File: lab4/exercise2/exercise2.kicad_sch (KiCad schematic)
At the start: 10 parts, among them J1 Conn_01x02_Male, U1 NE555D

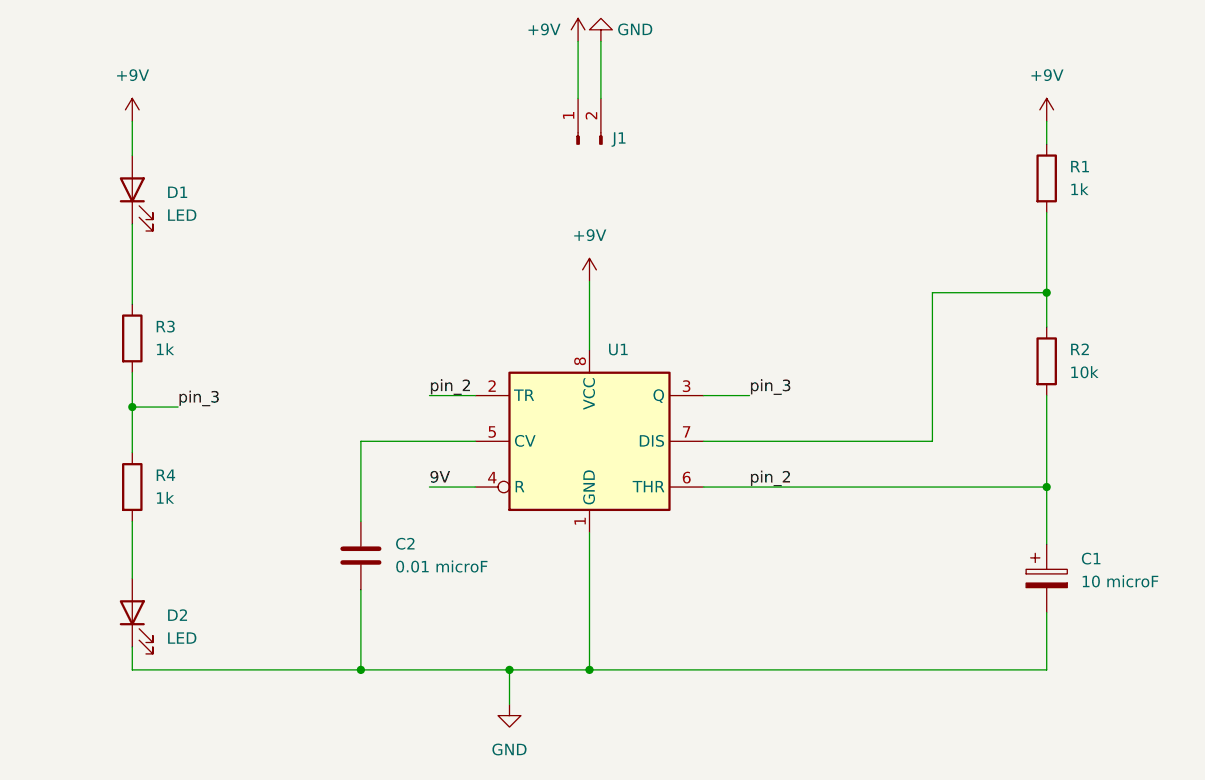
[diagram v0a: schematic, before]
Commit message: PCB layout
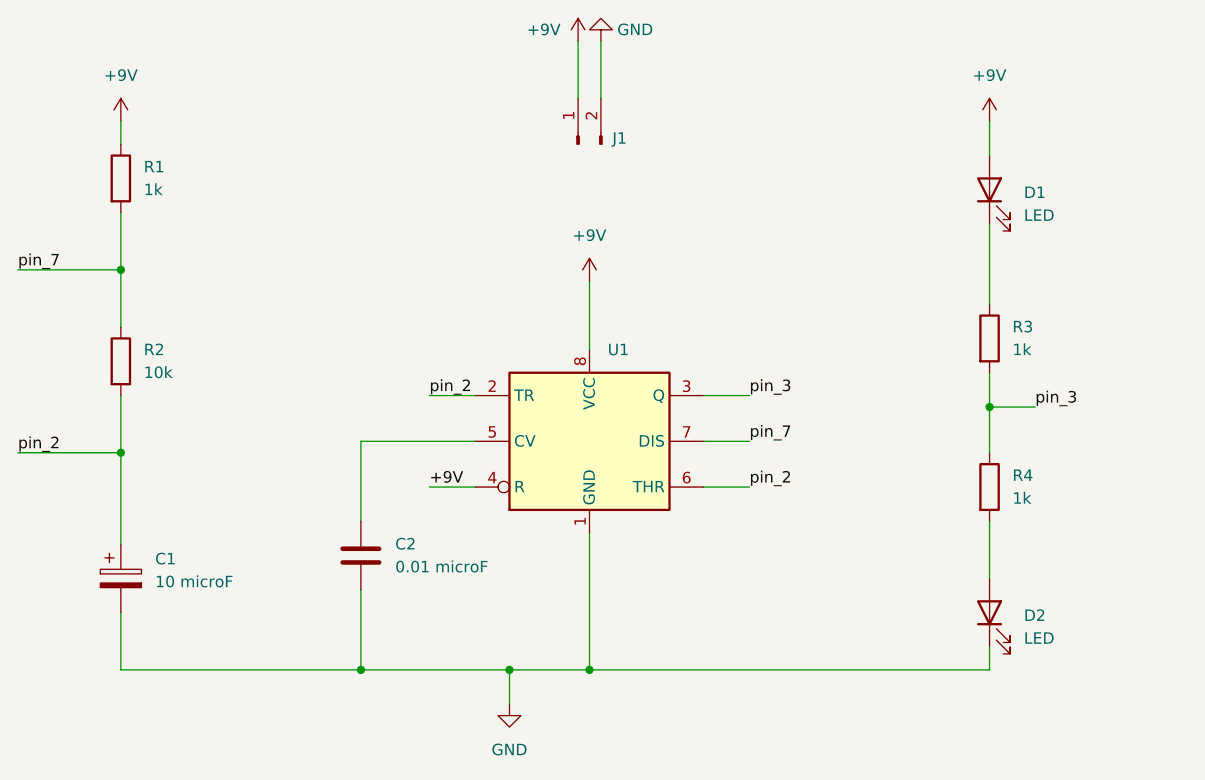
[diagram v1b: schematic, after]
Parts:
- C1: footprint (none) -> Capacitor_Tantalum_SMD:CP_EIA-3216-18_Kemet-A_Pad1.58x1.35mm_HandSolder
- C2: footprint (none) -> Capacitor_SMD:C_0805_2012Metric_Pad1.18x1.45mm_HandSolder
- D1, D2: footprint (none) -> LED_SMD:LED_1206_3216Metric_Pad1.42x1.75mm_HandSolder
- J1: footprint (none) -> TerminalBlock:TerminalBlock_bornier-2_P5.08mm
- R1, R2, R3, R4: footprint (none) -> Resistor_SMD:R_0805_2012Metric_Pad1.20x1.40mm_HandSolder
- U1: footprint Package_SO:SOIC-8_3.9x4.9mm_P1.27mm -> Package_SO:SOIC-8-1EP_3.9x4.9mm_P1.27mm_EP2.29x3mm
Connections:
- net 9V is gone; now on net +9V: U1.4 (R)
- net pin_7: now reaches R1.2, R2.1, U1.7 (DIS)
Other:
- moved on the sheet: C1, D1, D2, R1, R2, R3, R4
